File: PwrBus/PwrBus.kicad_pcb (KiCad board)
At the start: 2 copper layers, 149.9 x 25.4 mm, 16 parts, among them J1 Screw_Terminal_01x02, J10 Screw_Terminal_01x02, J2 Screw_Terminal_01x02, J3 Screw_Terminal_01x02, J4 Screw_Terminal_01x02, J5 Screw_Terminal_01x02, J6 Screw_Terminal_01x02, J7 Screw_Terminal_01x02, J8 Screw_Terminal_01x02, J9 Screw_Terminal_01x02, Q1 IRLML5203

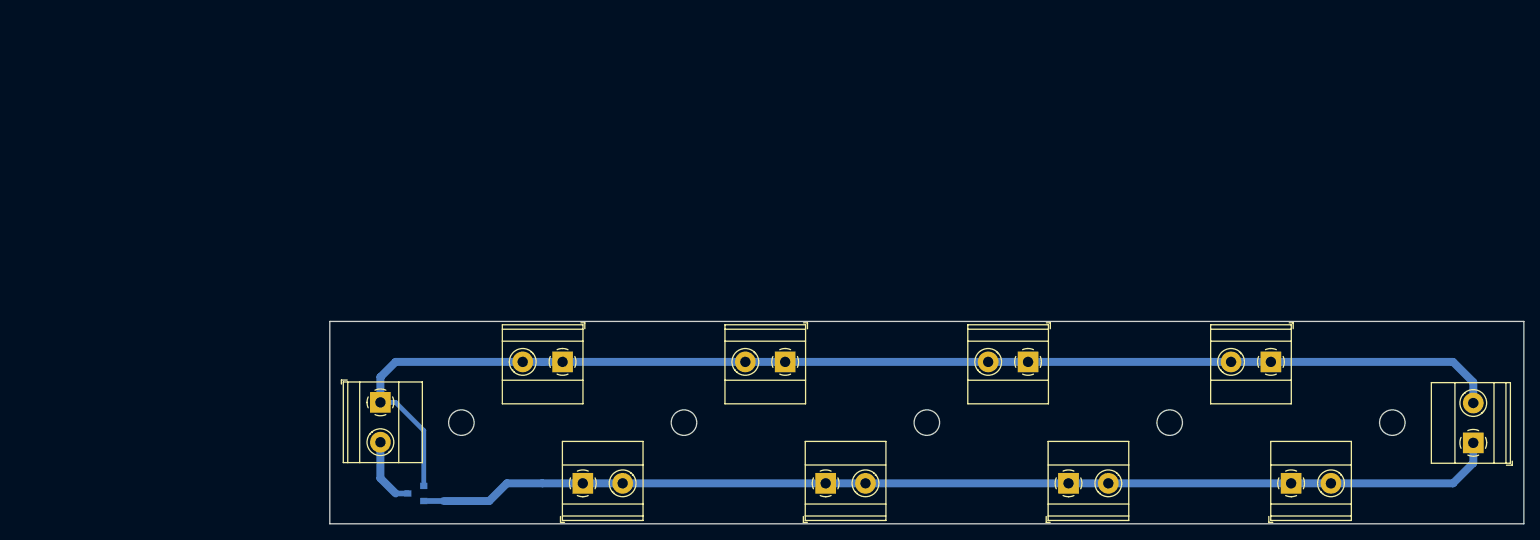
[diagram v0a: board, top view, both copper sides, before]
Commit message: Power bus is ready
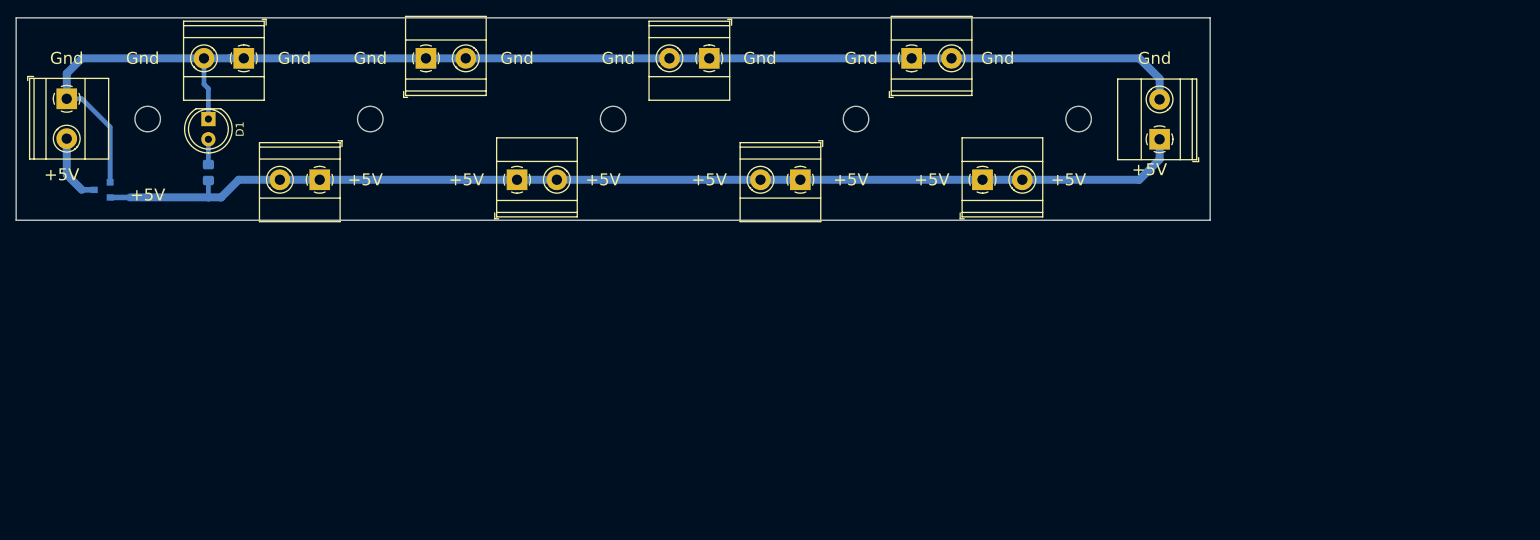
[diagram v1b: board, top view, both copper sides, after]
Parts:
- added D1: LED, LED_THT:LED_D5.0mm, F.Cu at (36.8, 25.4)
- added R1: 1k, Resistor_SMD:R_0805_2012Metric_Pad1.20x1.40mm_HandSolder, B.Cu at (36.8, 32.1)
- moved J9 59.0 mm to (125.1, 17.8), turned to 0 degrees
- moved J5 59.0 mm to (64.1, 17.8), turned to 0 degrees
- moved J3 55.2 mm to (41.3, 17.8)
- moved J7 55.2 mm to (99.7, 17.8)
- moved H3 54.8 mm to (87.6, 25.4)
- moved J1 54.8 mm to (19.1, 22.9)
- moved J10 54.8 mm to (156.2, 27.9)
- moved Q1 54.8 mm to (23.5, 34.3)
- moved H1 54.8 mm to (29.2, 25.4)
- moved H2 54.8 mm to (57.1, 25.4)
- moved H4 54.8 mm to (118.1, 25.4)
- moved H5 54.8 mm to (146.1, 25.4)
- moved J4 54.3 mm to (75.6, 33.0)
- moved J8 54.3 mm to (134.0, 33.0)
- moved J6 50.8 mm to (111.1, 33.0), turned to 180 degrees
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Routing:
- net GND: track 158.6 -> 166.5 mm
- net Net-(D1-Pad2): track 0.00 -> 3.17 mm
- net VCC: track 136.1 -> 138.3 mm
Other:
- board text added: "+5V"
- board text added: "Gnd"
